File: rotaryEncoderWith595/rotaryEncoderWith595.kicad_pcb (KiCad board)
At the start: 2 copper layers, 68 parts, among them J1 OUTCON, SW1 ROTENC, SW2 ROTENC, SW3 ROTENC, SW4 ROTENC, SW5 IN, SW6 IN, SW7 IN, SW8 IN, U1 74HC165, U2 74HC595, U3 74HC165, U4 74HC595

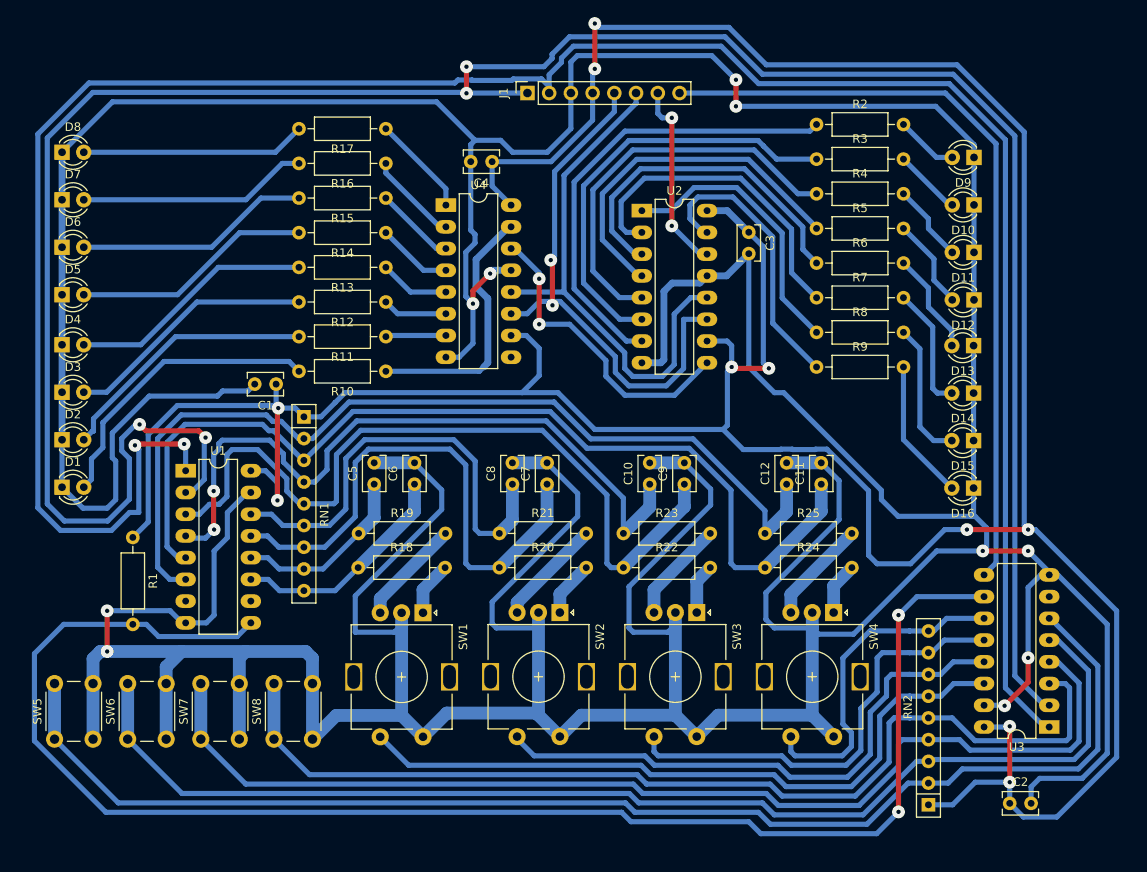
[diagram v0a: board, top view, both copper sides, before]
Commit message: finish route and generate pdf
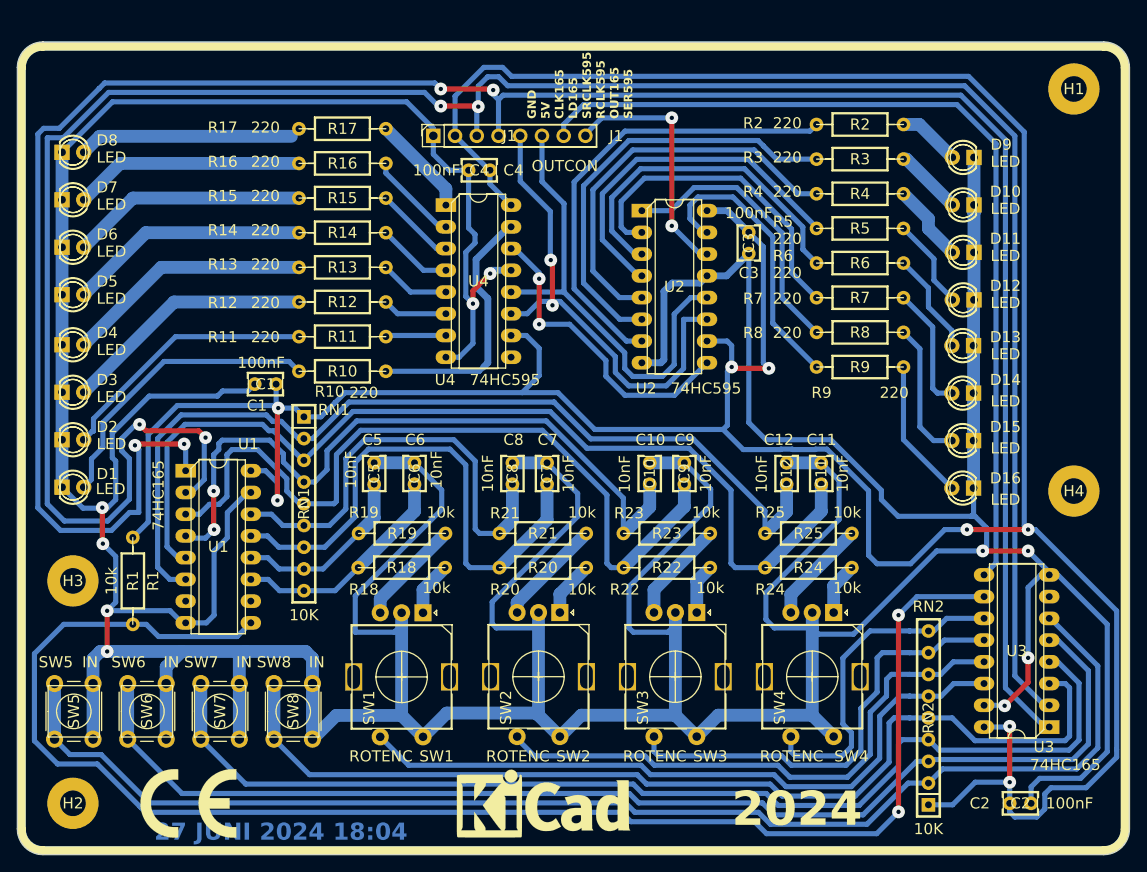
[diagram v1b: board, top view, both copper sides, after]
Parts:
- added H1: MountingHole_Pad, MountingHole:MountingHole_3mm_Pad, F.Cu at (211.0, 52.5)
- added H2: MountingHole_Pad, MountingHole:MountingHole_3mm_Pad, F.Cu at (94.0, 136.0)
- added H3: MountingHole_Pad, MountingHole:MountingHole_3mm_Pad, F.Cu at (94.0, 110.0)
- added H4: MountingHole_Pad, MountingHole:MountingHole_3mm_Pad, F.Cu at (211.0, 99.5)
- added REF**: CE-Logo_11.2x8mm_SilkScreen, Symbol:CE-Logo_11.2x8mm_SilkScreen, F.Cu at (107.5, 136.0)
- added REF**: KiCad-Logo_8mm_SilkScreen, Symbol:KiCad-Logo_8mm_SilkScreen, F.Cu at (149.0, 136.0)
- moved J1 12.1 mm to (136.1, 58.0)
- moved C4 1.03 mm to (142.8, 62.0)
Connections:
- J1 pad 1: /CLK165 -> GND
- J1 pad 2: /LD165 -> +5V
- J1 pad 3: GND -> /CLK165
- J1 pad 4: +5V -> /LD165
- J1 pad 7: /SER595 -> /OUT165
- J1 pad 8: /OUT165 -> /SER595
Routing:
- net GND: track 807.8 -> 781.9 mm
- net /OUT165: track 90.4 -> 105.7 mm
- net /RCLK595: track 62.1 -> 54.7 mm
- net /CLK165: track 281.3 -> 274.4 mm
- net /SER595: track 22.4 -> 29.2 mm
- net /SRCLK595: track 63.7 -> 57.1 mm
- net /LD165: track 270.9 -> 268.8 mm, vias 2 -> 4
- net +5V: track 406.5 -> 408.0 mm, vias 10 -> 8
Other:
- board outline added: 130 x 95 mm
- board text added: "2024"
- board text added: "27 JUNI 2024 18:04"
- board text added: "GND 5V CLK165 LD165 SRCLK595 RCLK595 OUT165 SER595"
